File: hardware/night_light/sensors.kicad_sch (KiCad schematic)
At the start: 10 parts, among them J1 RDB223, U4 LMV321

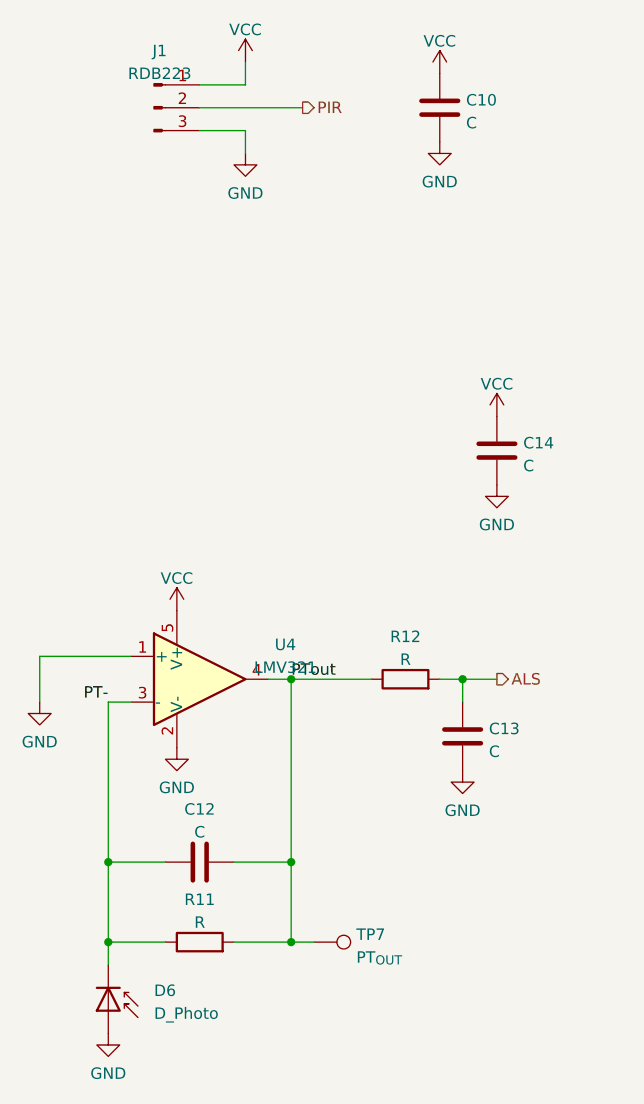
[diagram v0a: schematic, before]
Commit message: night light ready
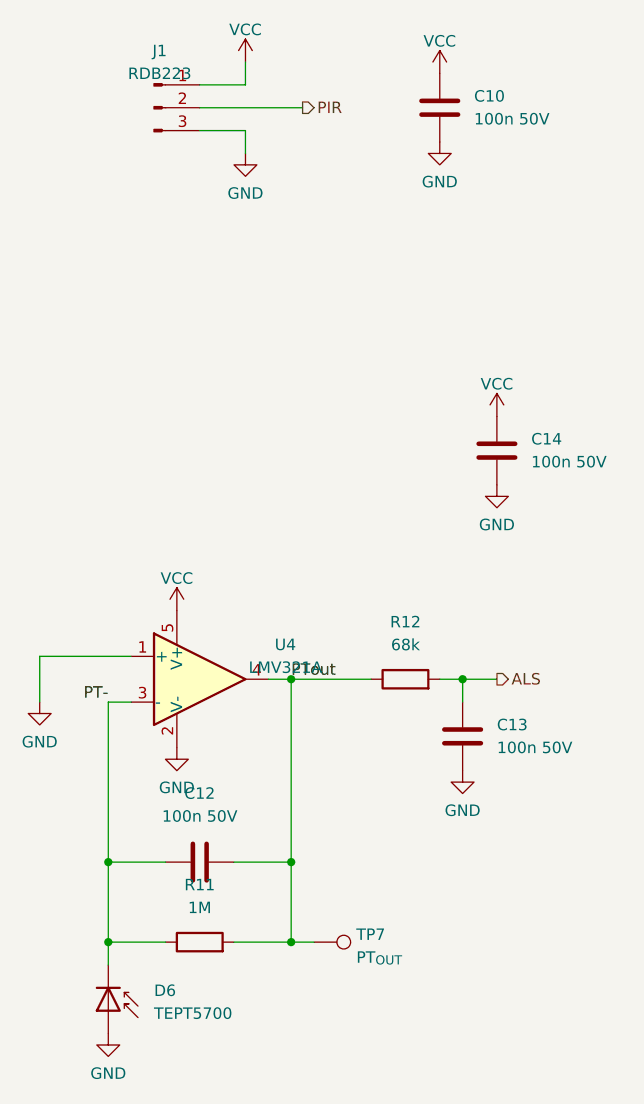
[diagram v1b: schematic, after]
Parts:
- C10, C12, C13, C14: value C -> 100n 50V
- D6: value D_Photo -> TEPT5700
- R11: value R -> 1M
- R12: value R -> 68k
- U4: value LMV321 -> LMV321A
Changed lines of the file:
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@@
   (symbol (lib_id "Device:C") (at 146.05 76.2 0) (unit 1)
     (in_bom yes) (on_board yes) (dnp no) (fields_autoplaced)
-    (property "Reference" "C10" (at 148.971 75.3653 0)
-      (effects (font (size 1.27 1.27)) (justify left))
-    )
-    (property "Value" "C" (at 148.971 77.9022 0)
+    (property "Reference" "C10" (at 149.86 74.93 0)
+      (effects (font (size 1.27 1.27)) (justify left))
+    )
+    (property "Value" "100n 50V" (at 149.86 77.47 0)
       (effects (font (size 1.27 1.27)) (justify left))
     )
@@
       (effects (font (size 1.27 1.27)) hide)
     )
+    (property "LCSC Part #" "" (at 146.05 76.2 0)
+      (effects (font (size 1.27 1.27)) hide)
+    )
     (pin "1")
     (pin "2")
@@
   (symbol (lib_id "Device:C") (at 152.4 114.3 0) (unit 1)
     (in_bom yes) (on_board yes) (dnp no) (fields_autoplaced)
-    (property "Reference" "C14" (at 155.321 113.4653 0)
-      (effects (font (size 1.27 1.27)) (justify left))
-    )
-    (property "Value" "C" (at 155.321 116.0022 0)
+    (property "Reference" "C14" (at 156.21 113.03 0)
+      (effects (font (size 1.27 1.27)) (justify left))
+    )
+    (property "Value" "100n 50V" (at 156.21 115.57 0)
       (effects (font (size 1.27 1.27)) (justify left))
     )
@@
       (effects (font (size 1.27 1.27)) hide)
     )
+    (property "LCSC Part #" "" (at 152.4 114.3 0)
+      (effects (font (size 1.27 1.27)) hide)
+    )
     (pin "1")
     (pin "2")
@@
       (effects (font (size 1.27 1.27)) (justify left))
     )
-    (property "Value" "D_Photo" (at 114.3 176.8475 90)
+    (property "Value" "TEPT5700" (at 114.3 176.8475 90)
       (effects (font (size 1.27 1.27)) (justify left))
     )
@@
     )
     (property "Datasheet" "~" (at 109.22 175.26 0)
+      (effects (font (size 1.27 1.27)) hide)
+    )
+    (property "LCSC Part #" "" (at 109.22 176.53 0)
       (effects (font (size 1.27 1.27)) hide)
     )
@@
       (effects (font (size 1.27 1.27)))
     )
-    (property "Value" "LMV321" (at 128.8997 138.4102 0)
+    (property "Value" "LMV321A" (at 128.8997 138.4102 0)
       (effects (font (size 1.27 1.27)))
     )
@@
       (effects (font (size 1.27 1.27)) hide)
     )
+    (property "LCSC Part #" "" (at 119.38 139.7 0)
+      (effects (font (size 1.27 1.27)) hide)
+    )
     (pin "2")
     (pin "5")
@@
   (symbol (lib_id "Device:C") (at 148.59 146.05 180) (unit 1)
     (in_bom yes) (on_board yes) (dnp no) (fields_autoplaced)
-    (property "Reference" "C13" (at 151.511 145.2153 0)
+    (property "Reference" "C13" (at 152.4 144.78 0)
       (effects (font (size 1.27 1.27)) (justify right))
     )
-    (property "Value" "C" (at 151.511 147.7522 0)
+    (property "Value" "100n 50V" (at 152.4 147.32 0)
       (effects (font (size 1.27 1.27)) (justify right))
     )
@@
       (effects (font (size 1.27 1.27)) hide)
     )
+    (property "LCSC Part #" "" (at 148.59 146.05 0)
+      (effects (font (size 1.27 1.27)) hide)
+    )
     (pin "1")
     (pin "2")
@@
       (effects (font (size 1.27 1.27)) hide)
     )
+    (property "LCSC Part #" "" (at 114.3 76.2 0)
+      (effects (font (size 1.27 1.27)) hide)
+    )
     (pin "1")
     (pin "2")
@@
   (symbol (lib_id "Device:R") (at 142.24 139.7 90) (unit 1)
     (in_bom yes) (on_board yes) (dnp no) (fields_autoplaced)
-    (property "Reference" "R12" (at 142.24 134.9842 90)
-      (effects (font (size 1.27 1.27)))
-    )
-    (property "Value" "R" (at 142.24 137.5211 90)
+    (property "Reference" "R12" (at 142.24 133.35 90)
+      (effects (font (size 1.27 1.27)))
+    )
+    (property "Value" "68k" (at 142.24 135.89 90)
       (effects (font (size 1.27 1.27)))
     )
@@
       (effects (font (size 1.27 1.27)) hide)
     )
+    (property "LCSC Part #" "" (at 142.24 139.7 0)
+      (effects (font (size 1.27 1.27)) hide)
+    )
     (pin "1")
     (pin "2")
@@
   (symbol (lib_id "Device:R") (at 119.38 168.91 90) (unit 1)
     (in_bom yes) (on_board yes) (dnp no) (fields_autoplaced)
-    (property "Reference" "R11" (at 119.38 164.1942 90)
-      (effects (font (size 1.27 1.27)))
-    )
-    (property "Value" "R" (at 119.38 166.7311 90)
+    (property "Reference" "R11" (at 119.38 162.56 90)
+      (effects (font (size 1.27 1.27)))
+    )
+    (property "Value" "1M" (at 119.38 165.1 90)
       (effects (font (size 1.27 1.27)))
     )
@@
       (effects (font (size 1.27 1.27)) hide)
     )
+    (property "LCSC Part #" "" (at 119.38 168.91 0)
+      (effects (font (size 1.27 1.27)) hide)
+    )
     (pin "1")
     (pin "2")
@@
   (symbol (lib_id "Device:C") (at 119.38 160.02 90) (unit 1)
     (in_bom yes) (on_board yes) (dnp no) (fields_autoplaced)
-    (property "Reference" "C12" (at 119.38 154.1612 90)
-      (effects (font (size 1.27 1.27)))
-    )
-    (property "Value" "C" (at 119.38 156.6981 90)
+    (property "Reference" "C12" (at 119.38 152.4 90)
+      (effects (font (size 1.27 1.27)))
+    )
+    (property "Value" "100n 50V" (at 119.38 154.94 90)
       (effects (font (size 1.27 1.27)))
     )
@@
       (effects (font (size 1.27 1.27)) hide)
     )
+    (property "LCSC Part #" "" (at 119.38 160.02 0)
+      (effects (font (size 1.27 1.27)) hide)
+    )
     (pin "1")
     (pin "2")
@@
       (effects (font (size 1.27 1.27)) hide)
     )
+    (property "LCSC Part #" "" (at 132.08 168.91 0)
+      (effects (font (size 1.27 1.27)) hide)
+    )

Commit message: various
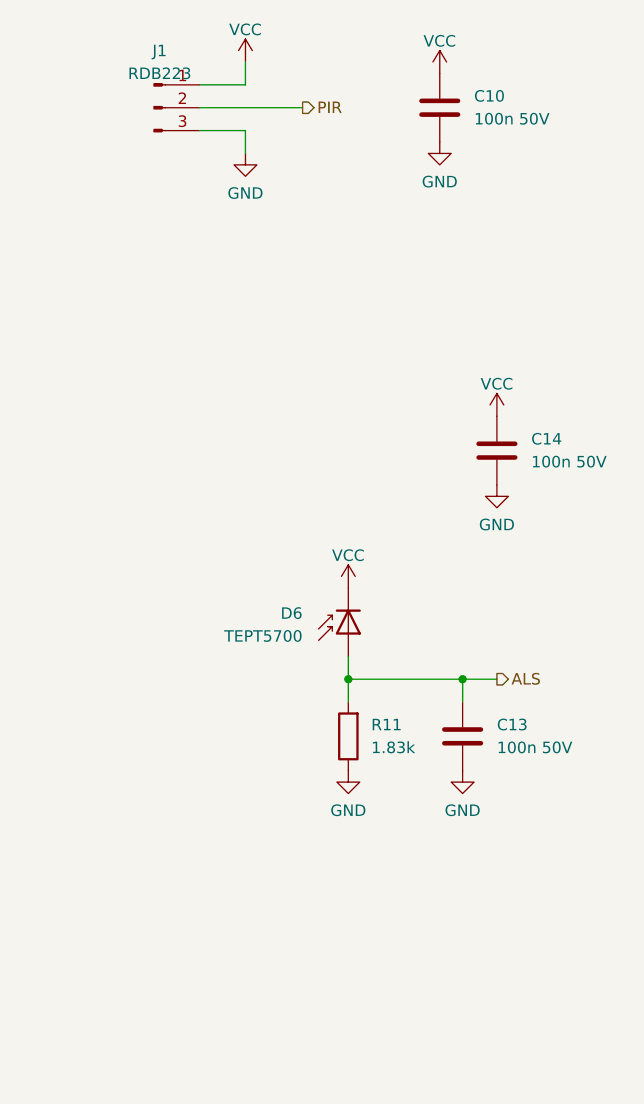
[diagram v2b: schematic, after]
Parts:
- removed C12: 100n 50V, Capacitor_SMD:C_0603_1608Metric, symbol Device:C
- removed R12: 68k, Resistor_SMD:R_0603_1608Metric, symbol Device:R
- removed TP7: PT_{OUT}, prj_lib:TestPoint_THTPad_D1.0mm_Drill0.5mm, symbol Connector:TestPoint
- removed U4: LMV321A, Package_TO_SOT_SMD:SOT-23-5, symbol Amplifier_Operational:LMV321
- C10, C13, C14: LCSC (none) -> C14663
- D6: footprint LED_THT:LED_D3.0mm_Clear -> LED_THT:LED_D3.0mm_FlatTop
- J1: LCSC (none) -> C879408
- R11: value 1M -> 1.83k
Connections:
- net PTout is gone; now on net ALS: R11.2
- net ALS: now also D6.2 (A)
- net GND: now also R11.1; no longer D6.2 (A)
- net VCC: now also D6.1 (K)
- removed net PT-: D6.1 (K), R11.1
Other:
- moved on the sheet: D6, R11
